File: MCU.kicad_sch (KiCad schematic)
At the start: 28 parts, among them J1 USB_C_Receptacle_USB2.0_16P, J2 FTSH-105-01-L-DV-K-A, U1 STM32H743VITx, Y1 Crystal_GND24

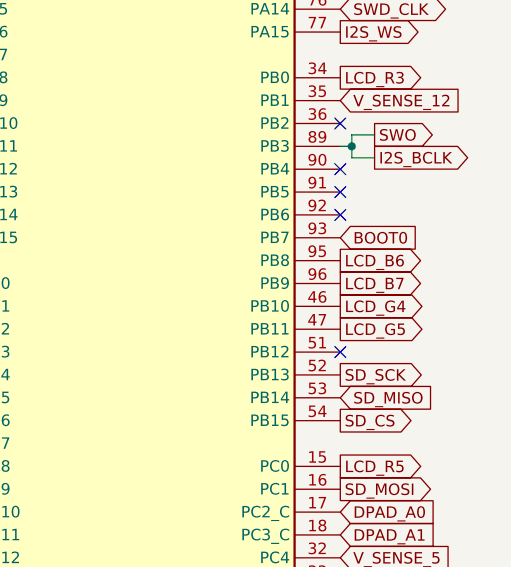
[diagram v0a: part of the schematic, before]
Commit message: full preliminary layout
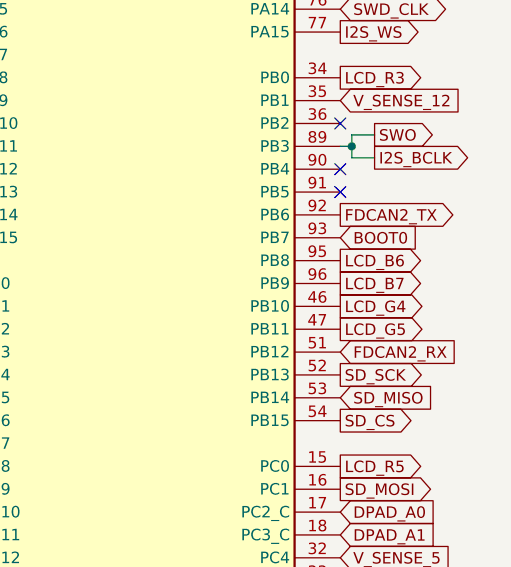
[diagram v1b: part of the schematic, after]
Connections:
- net FDCAN2_RX: now reaches U1.51 (PB12)
- net FDCAN2_TX: now reaches U1.92 (PB6)
- no-connect marks 30 -> 28
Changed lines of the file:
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@@
-	)
-	(no_connect
-		(at 261.62 85.09)
 	)
 	(no_connect
@@
 	(no_connect
 		(at 261.62 125.73)
-	)
-	(no_connect
-		(at 261.62 100.33)
 	)
 	(no_connect
@@
 		)
 	)
+	(global_label "FDCAN2_RX"
+		(shape input)
+		(at 261.62 100.33 0)
+		(fields_autoplaced yes)
+		(effects
+			(font
+				(size 1.27 1.27)
+			)
+			(justify left)
+		)
+		(property "Intersheetrefs" "${INTERSHEET_REFS}"
+			(at 275.3095 100.33 0)
+			(effects
+				(font
+					(size 1.27 1.27)
+				)
+				(justify left)
+				(hide yes)
+			)
+		)
+	)
 	(global_label "BOOT0"
 		(shape input)
@@
 			(effects
 				(font
+					(size 1.27 1.27)
+				)
+				(justify left)
+				(hide yes)
+			)
+		)
+	)
+	(global_label "FDCAN2_TX"
+		(shape output)
+		(at 261.62 85.09 0)
+		(fields_autoplaced yes)
+		(effects
+			(font
+				(size 1.27 1.27)
+			)
+			(justify left)
+		)
+		(property "Intersheetrefs" "${INTERSHEET_REFS}"
+			(at 275.0071 85.09 0)
+			(effects
+				(font
